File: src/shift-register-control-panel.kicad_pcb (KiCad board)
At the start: 2 copper layers, 69.2 x 41.8 mm, 34 parts, among them J1 Conn_01x08, J2 USB_A, SW1 INPUT, SW2 SHIFT, SW3 CLEAR, SW4 DISPLAY, U1 74HC595, U2 LM7805_TO220, U3 SN74LVC1G14

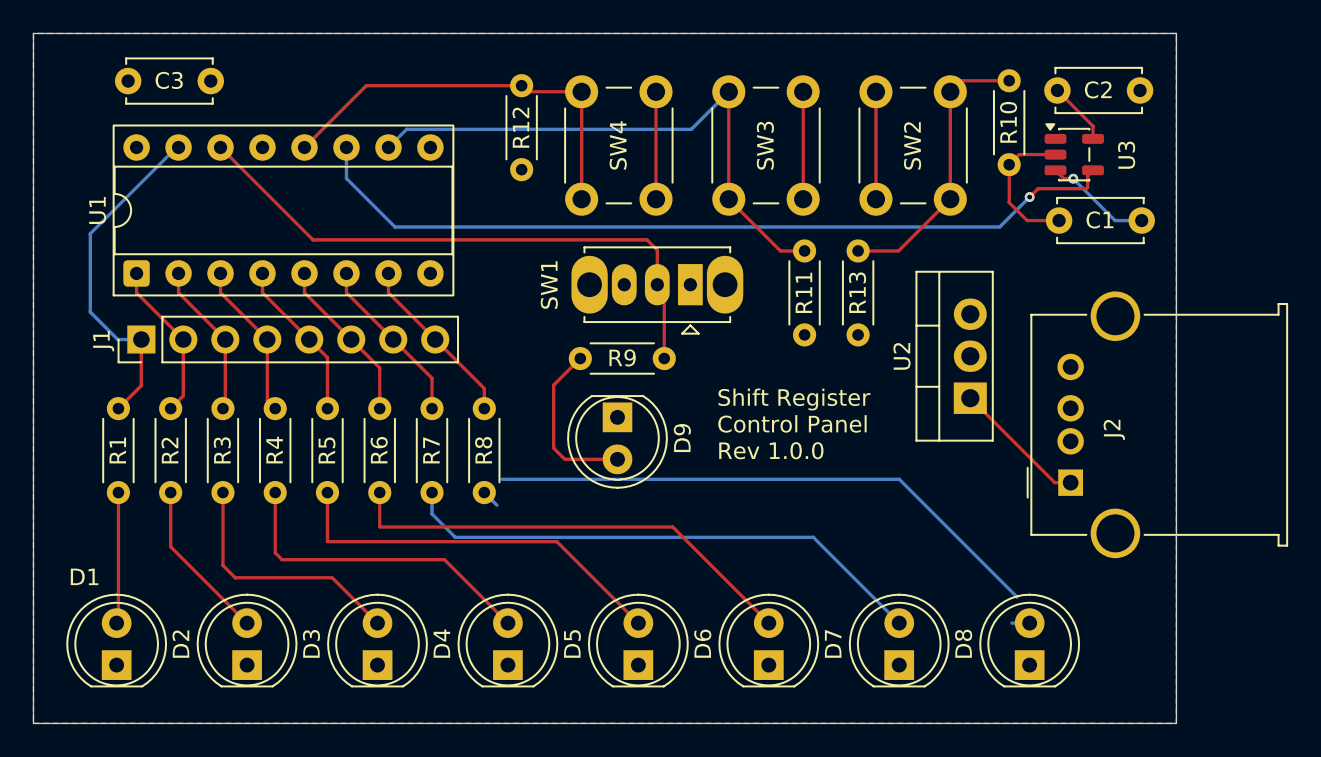
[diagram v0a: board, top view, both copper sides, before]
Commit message: updated with OSH Park DRC
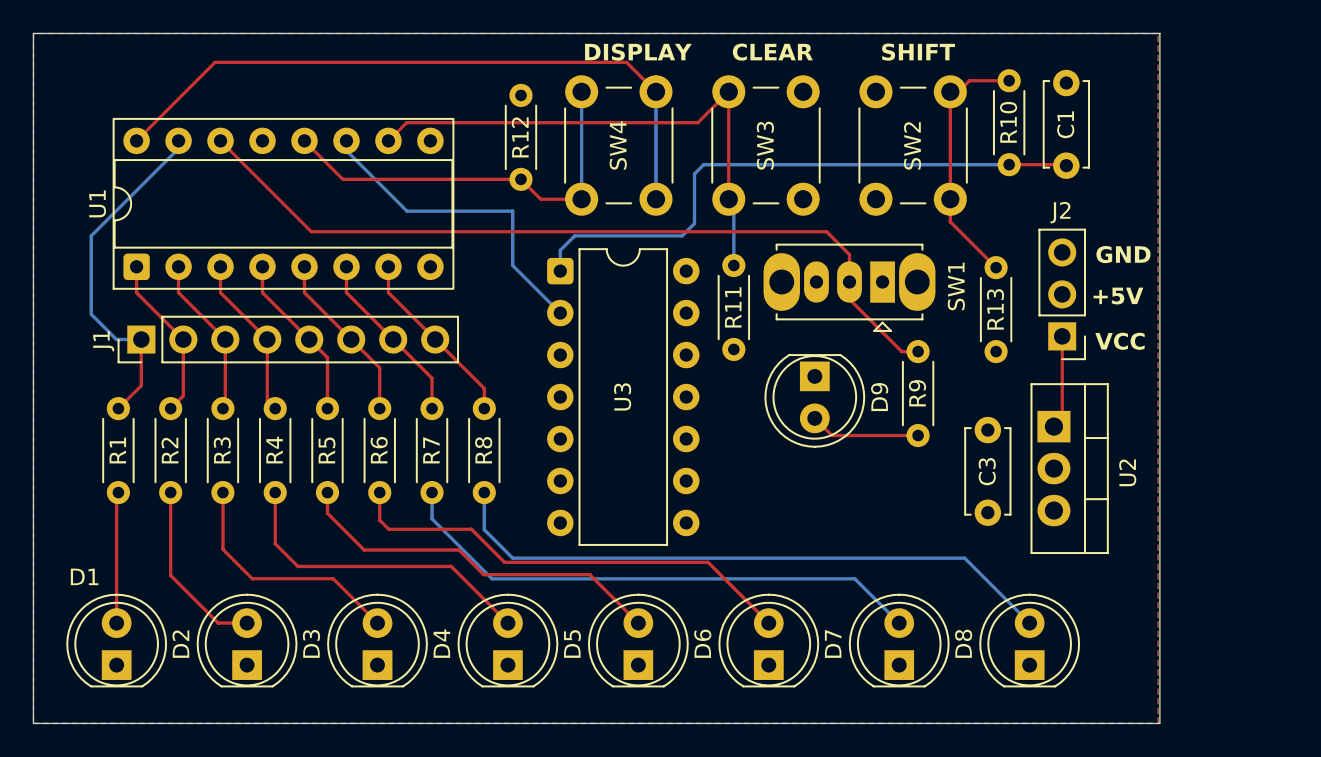
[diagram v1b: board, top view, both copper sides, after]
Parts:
- removed C2: 100 nF, Capacitor_THT:C_Disc_D5.0mm_W2.5mm_P5.00mm
- J2: value USB_A -> Conn_01x03; footprint Connector_USB:USB_A_Molex_67643_Horizontal -> Connector_PinHeader_2.54mm:PinHeader_1x03_P2.54mm_Vertical
- U2: value LM7805_TO220 -> LM7805
- U3: value SN74LVC1G14 -> 74HC14; footprint Package_TO_SOT_SMD:SOT-23-5 -> Package_DIP:DIP-14_W7.62mm
- moved C3 53.8 mm to (180.2, 103.8), turned to 90 degrees
- moved U3 31.9 mm to (154.4, 89.1)
- moved R9 15.4 mm to (176.0, 94.0), turned to -90 degrees
- moved D9 12.2 mm to (169.8, 95.5)
- moved SW1 11.6 mm to (173.9, 89.8)
- moved J2 8.86 mm to (184.8, 93.1), turned to 180 degrees
- moved R13 8.41 mm to (180.8, 88.9)
- moved R12 5.67 mm to (152.0, 83.6), turned to 90 degrees
- moved U2 5.34 mm to (184.2, 98.5), turned to -90 degrees
- moved R11 4.37 mm to (164.9, 93.9)
- moved C1 3.35 mm to (185.0, 82.8), turned to 90 degrees
- moved U1 0.40 mm to (128.7, 88.9)
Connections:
- C3 pad 1: GND -> +5V
- C3 pad 2: +5V -> GND
- J2 pad 2: unconnected-(J2-D--Pad2) -> +5V
- J2 pad 3: unconnected-(J2-D+-Pad3) -> GND
- U3 pad 1: unconnected-(U3-NC-Pad1) -> Net-(C1-Pad1)
- U3 pad 2: Net-(C1-Pad1) -> Net-(U1-SRCLK)
- U3 pad 3: GND -> unconnected-(U3-Pad3)
- U3 pad 4: Net-(U1-SRCLK) -> unconnected-(U3-Pad4)
- U3 pad 5: +5V -> unconnected-(U3-Pad5)
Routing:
- net Net-(U1-SRCLK): track 50.1 -> 19.5 mm, vias 1 -> 0
- net +5V: track 10.3 -> 40.6 mm
- net Net-(C1-Pad1): track 8.82 -> 35.8 mm
- net GND: track 19.5 -> 0.00 mm, vias 1 -> 0
- net Net-(SW1-B): track 35.7 -> 49.1 mm
- net Net-(D9-A): track 10.2 -> 6.68 mm
- net VCC: track 8.19 -> 5.67 mm
- net Net-(U1-~{SRCLR}): track 34.4 -> 32.5 mm
- net Net-(R10-Pad1): track 17.2 -> 15.6 mm
- net Net-(D8-A): track 36.3 -> 37.6 mm
- net Net-(D2-A): track 9.81 -> 10.8 mm
- net Net-(D5-A): track 23.8 -> 22.8 mm
- net Net-(D3-A): track 15.2 -> 14.6 mm
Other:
- board size 69.2 x 41.8 mm -> 68.2 x 41.8 mm
- rule pad_to_mask_clearance: 0 -> 0.0508
- board text added: "+5V"
- board text added: "CLEAR"
- board text added: "DISPLAY"
- board text added: "GND"
- board text added: "SHIFT"
- board text added: "VCC"
- board text removed: "Shift Register Control Panel Rev 1.0.0"
